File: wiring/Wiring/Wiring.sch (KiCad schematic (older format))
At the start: 7 parts, among them U1 MAIN, U2 E, U3 F, U4 G

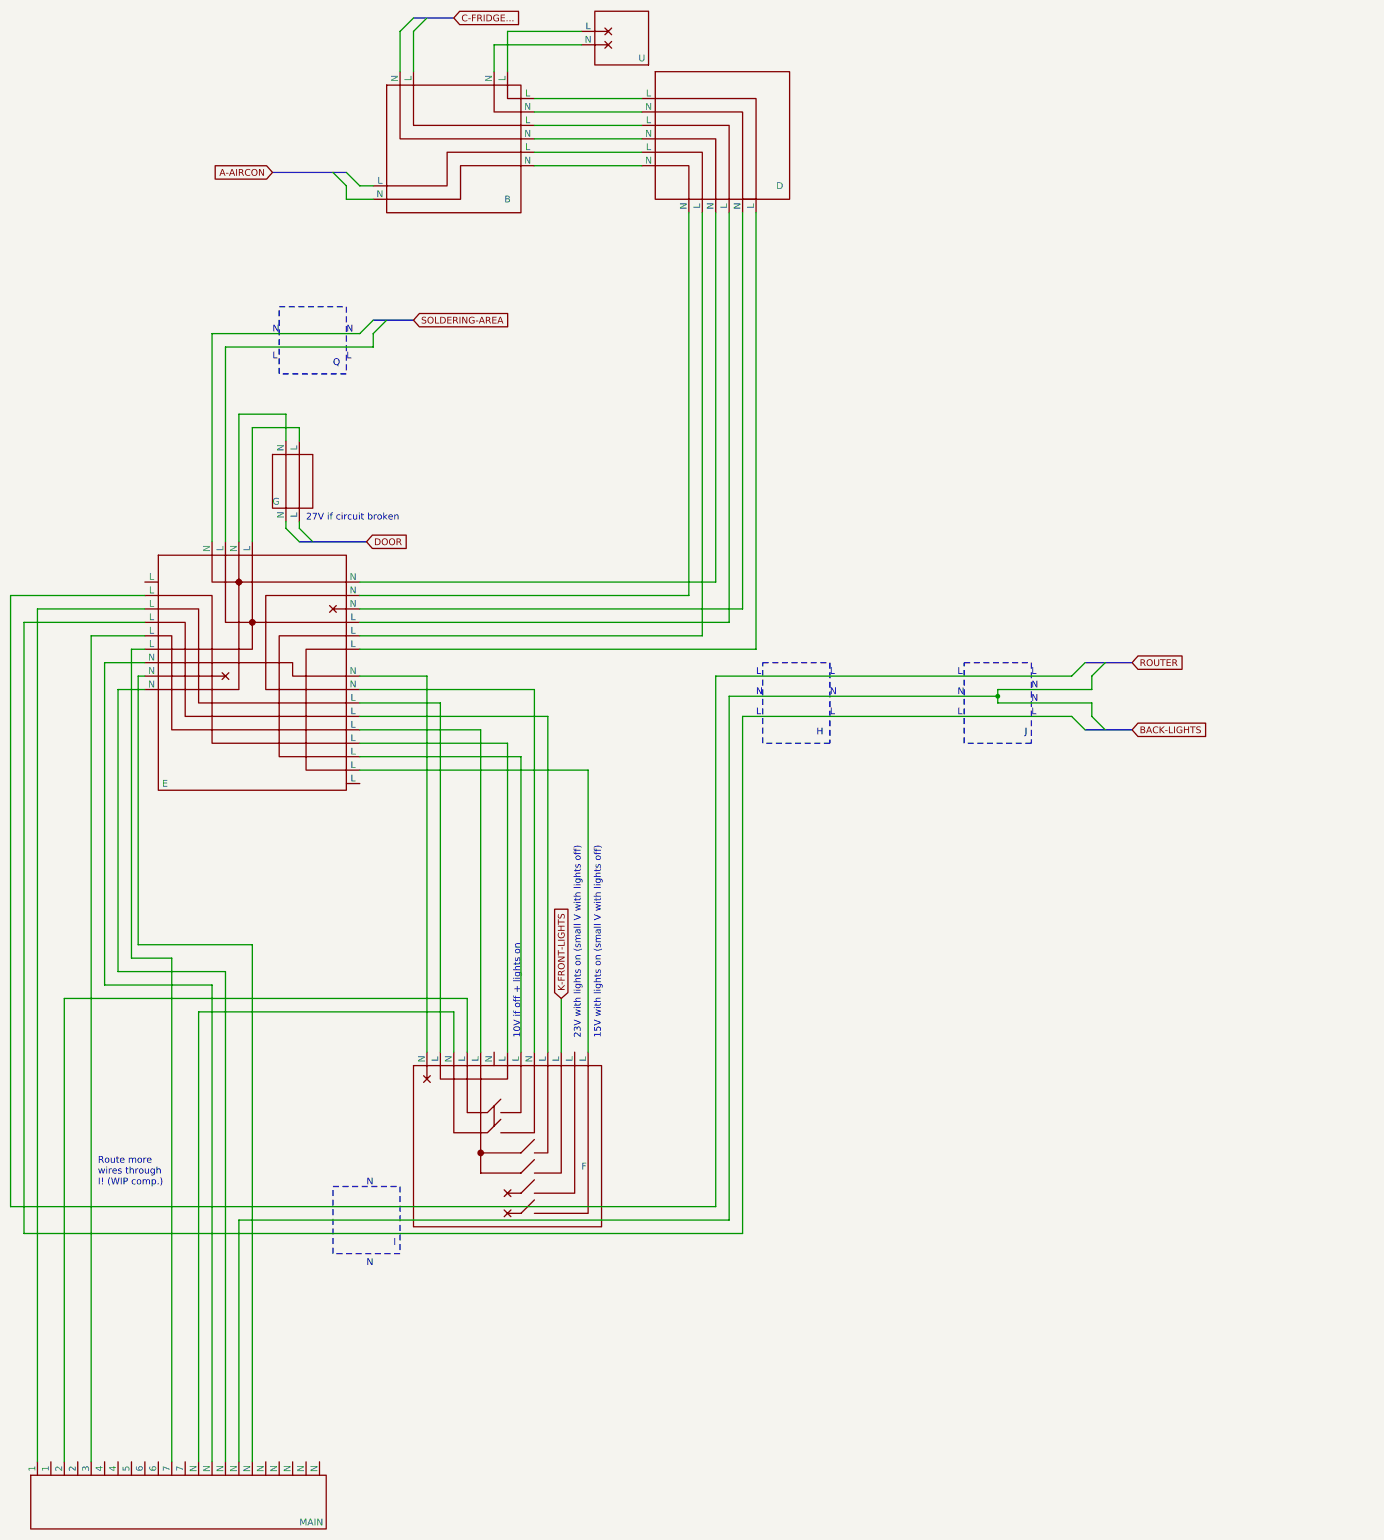
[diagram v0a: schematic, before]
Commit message: Add V
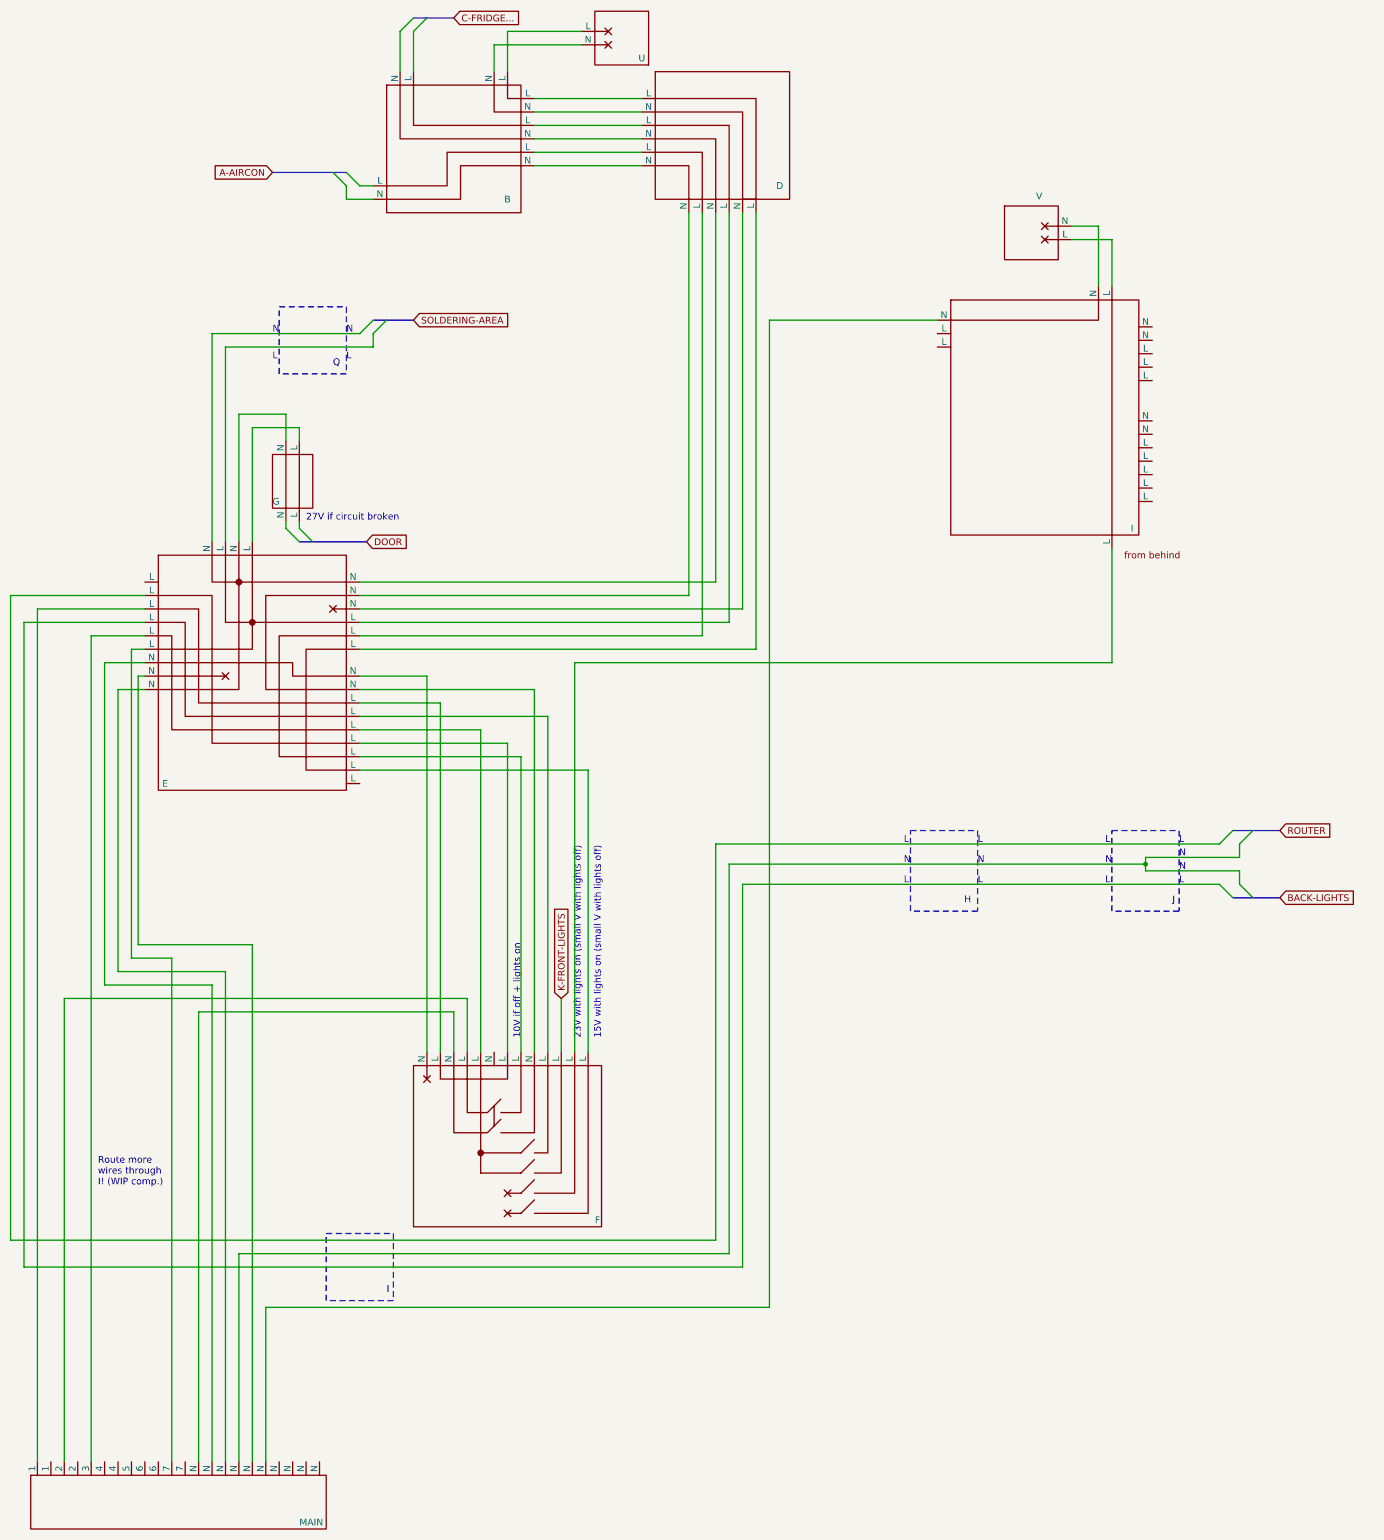
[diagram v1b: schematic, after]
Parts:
- added U?: I, symbol Wiring:I
- added U?: V, symbol Wiring:V
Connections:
- net at U3.12 (L): now also U?.~ (N)
- net at U1.~ (N): now also U?.16 (N)
- net at U?.~ (N): now also U?.12 (L)
- new net: U2.14 (L), U?.12 (L)
- new net: U?.10 (N), U?.8 (N) (x2)
- new net: U?.12 (L), U?.9 (L) (x2)
- new net: U?.10 (N), U?.~ (N)
- new net: U?.12 (L), U?.~ (N)
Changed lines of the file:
@@
 P 12550 8850
 F 0 "U3" H 13178 8929 50  0001 L CNN
-F 1 "F" H 13150 8450 50  0000 L CNN
+F 1 "F" H 13250 8050 50  0000 L CNN
 F 2 "Package_DFN_QFN:DFN-8-1EP_4x4mm_P0.8mm_EP2.5x3.6mm" H 12500 9000 50  0001 C CNN
 F 3 "" H 12500 9000 50  0001 C CNN
@@
 27V if circuit broken
 Wire Notes Line
-	14500 5500 15000 5500
-Wire Notes Line
-	15000 5500 15000 6100
-Wire Notes Line
-	14500 6100 14500 5500
-Text Notes 14900 6050 0    50   ~ 0
+	15600 6750 16100 6750
+Wire Notes Line
+	16100 6750 16100 7350
+Wire Notes Line
+	15600 7350 15600 6750
+Text Notes 16000 7300 0    50   ~ 0
 H
 Wire Notes Line
-	16000 5500 16500 5500
-Wire Notes Line
-	16500 5500 16500 6100
-Wire Notes Line
-	16500 6100 16000 6100
-Wire Notes Line
-	16000 6100 16000 5500
-Text Notes 16450 6050 0    50   ~ 0
+	17100 6750 17600 6750
+Wire Notes Line
+	17600 6750 17600 7350
+Wire Notes Line
+	17600 7350 17100 7350
+Wire Notes Line
+	17100 7350 17100 6750
+Text Notes 17550 7300 0    50   ~ 0
 J
-Text GLabel 17250 5500 2    50   Input ~ 0
+Text GLabel 18350 6750 2    50   Input ~ 0
 ROUTER
 Entry Wire Line
-	16800 5600 16900 5500
-Wire Wire Line
-	16800 5600 14150 5600
-Wire Wire Line
-	14250 9650 14250 5750
-Entry Wire Line
-	17050 5500 16950 5600
-Wire Wire Line
-	16950 5700 16950 5600
-Wire Notes Line
-	11300 9400 11800 9400
-Wire Notes Line
-	11800 9900 11300 9900
-Wire Notes Line
-	11300 9900 11300 9400
-Text Notes 11750 9850 0    50   ~ 0
+	17900 6850 18000 6750
+Entry Wire Line
+	18150 6750 18050 6850
+Wire Wire Line
+	18050 6950 18050 6850
+Wire Notes Line
+	11250 9750 11750 9750
+Wire Notes Line
+	11750 10250 11250 10250
+Wire Notes Line
+	11250 10250 11250 9750
+Text Notes 11700 10200 0    50   ~ 0
 I
 Wire Wire Line
 	12900 5900 12900 8400
 Wire Notes Line
-	15000 6100 14500 6100
-Wire Wire Line
-	16250 5700 16950 5700
-Wire Wire Line
-	16250 5750 16250 5700
-Wire Wire Line
-	14250 5750 16250 5750
-Wire Wire Line
-	16250 5750 16250 5800
-Wire Wire Line
-	16250 5800 16950 5800
-Connection ~ 16250 5750
-Text Notes 16500 5600 0    50   ~ 0
-L
-Text Notes 16500 5700 0    50   ~ 0
-N
-Text Notes 16500 5800 0    50   ~ 0
-N
-Text Notes 16500 5900 0    50   ~ 0
-L
-Text Notes 15950 5600 0    50   ~ 0
-L
-Text Notes 15950 5750 0    50   ~ 0
-N
-Text Notes 15950 5900 0    50   ~ 0
-L
-Text Notes 15000 5600 0    50   ~ 0
-L
-Text Notes 15000 5900 0    50   ~ 0
-L
-Text Notes 15000 5750 0    50   ~ 0
-N
-Text Notes 14450 5750 0    50   ~ 0
-N
-Text Notes 14450 5600 0    50   ~ 0
-L
-Text Notes 14450 5900 0    50   ~ 0
-L
-Text Notes 11550 9400 0    50   ~ 0
-N
-Text Notes 11550 10000 0    50   ~ 0
-N
-Text GLabel 17250 6000 2    50   Input ~ 0
+	16100 7350 15600 7350
+Wire Wire Line
+	17350 6950 18050 6950
+Wire Wire Line
+	17350 7000 17350 6950
+Wire Wire Line
+	17350 7000 17350 7050
+Wire Wire Line
+	17350 7050 18050 7050
+Connection ~ 17350 7000
+Text Notes 17600 6850 0    50   ~ 0
+L
+Text Notes 17600 6950 0    50   ~ 0
+N
+Text Notes 17600 7050 0    50   ~ 0
+N
+Text Notes 17600 7150 0    50   ~ 0
+L
+Text Notes 17050 6850 0    50   ~ 0
+L
+Text Notes 17050 7000 0    50   ~ 0
+N
+Text Notes 17050 7150 0    50   ~ 0
+L
+Text Notes 16100 6850 0    50   ~ 0
+L
+Text Notes 16100 7150 0    50   ~ 0
+L
+Text Notes 16100 7000 0    50   ~ 0
+N
+Text Notes 15550 7000 0    50   ~ 0
+N
+Text Notes 15550 6850 0    50   ~ 0
+L
+Text Notes 15550 7150 0    50   ~ 0
+L
+Text GLabel 18350 7250 2    50   Input ~ 0
 BACK-LIGHTS
 Entry Wire Line
-	16800 5900 16900 6000
-Entry Wire Line
-	16950 5900 17050 6000
-Wire Wire Line
-	16950 5800 16950 5900
+	17900 7150 18000 7250
+Entry Wire Line
+	18050 7150 18150 7250
+Wire Wire Line
+	18050 7050 18050 7150
 Wire Wire Line
 	12300 8400 12300 8000
@@
 	10500 11450 10500 7800
 Wire Wire Line
-	10600 9650 10600 11450
+	10600 9900 10600 11450
 Wire Wire Line
 	9900 5600 9850 5600
@@
 	12900 5900 11500 5900
 Wire Wire Line
-	10600 9650 14250 9650
-Wire Wire Line
-	14350 5900 14350 9750
-Wire Wire Line
-	14350 5900 16800 5900
-Wire Wire Line
-	14150 5600 14150 9550
+	10600 9900 14250 9900
+Wire Wire Line
+	14350 7150 14350 10000
+Wire Wire Line
+	14150 6850 14150 9800
 Wire Wire Line
 	9900 5200 9000 5200
 Wire Wire Line
-	9000 5200 9000 9750
+	9000 5200 9000 10000
 Wire Wire Line
 	9900 5000 8900 5000
 Wire Wire Line
-	8900 5000 8900 9550
-Wire Notes Line
-	11800 9400 11800 9900
-Wire Wire Line
-	8900 9550 14150 9550
-Wire Wire Line
-	9000 9750 14350 9750
+	8900 5000 8900 9800
+Wire Notes Line
+	11750 9750 11750 10250
+Wire Wire Line
+	8900 9800 14150 9800
+Wire Wire Line
+	9000 10000 14350 10000
 Text Notes 9550 9400 0    50   ~ 0
 Route more\nwires through\nI! (WIP comp.)
@@
 Wire Wire Line
 	11500 5400 14450 5400
+$Comp
+L Wiring:I U?
+U 1 1 5EE80A79
+P 16600 3650
+F 0 "U?" H 17350 2700 50  0001 C CNN
+F 1 "I" H 17250 2800 50  0000 C CNN
+F 2 "" H 15900 3500 50  0001 C CNN
+F 3 "" H 15900 3500 50  0001 C CNN
+	1    16600 3650
+	1    0    0    -1
+$EndComp
+Wire Wire Line
+	14250 9900 14250 7000
+Wire Wire Line
+	13100 5500 17100 5500
+Wire Wire Line
+	17100 5500 17100 4650
+Wire Wire Line
+	13100 5500 13100 8400
+$Comp
+L Wiring:V U?
+U 1 1 5EE9031E
+P 16500 2300
+F 0 "U?" H 16350 2450 50  0001 C CNN
+F 1 "V" H 16558 2573 50  0000 C CNN
+F 2 "" H 15800 2150 50  0001 C CNN
+F 3 "" H 15800 2150 50  0001 C CNN
+	1    16500 2300
+	1    0    0    -1
+$EndComp
+Wire Wire Line
+	16800 2350 17100 2350
+Wire Wire Line
+	17100 2350 17100 2700
+Wire Wire Line
+	17000 2700 17000 2250
+Wire Wire Line
+	17000 2250 16800 2250
+Wire Wire Line
+	14550 2950 14550 10300
+Wire Wire Line
+	14550 10300 10800 10300
+Wire Wire Line
+	10800 10300 10800 11450
+Wire Wire Line
+	14150 6850 17900 6850
+Wire Wire Line
+	14250 7000 17350 7000
+Wire Wire Line
+	14350 7150 17900 7150
+Wire Wire Line
+	14550 2950 15800 2950
 Wire Bus Line
 	10850 1850 11400 1850
@@
 	11600 2950 11900 2950
 Wire Bus Line
-	16900 6000 17250 6000
+	18000 7250 18350 7250
 Wire Bus Line
-	16900 5500 17250 5500
+	18000 6750 18350 6750
 Wire Bus Line
 	11900 700  12200 700
